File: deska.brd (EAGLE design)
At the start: 64.4 x 69.8 mm, 17 parts, among them X1 JST-XH-03-PIN-LONG-PAD

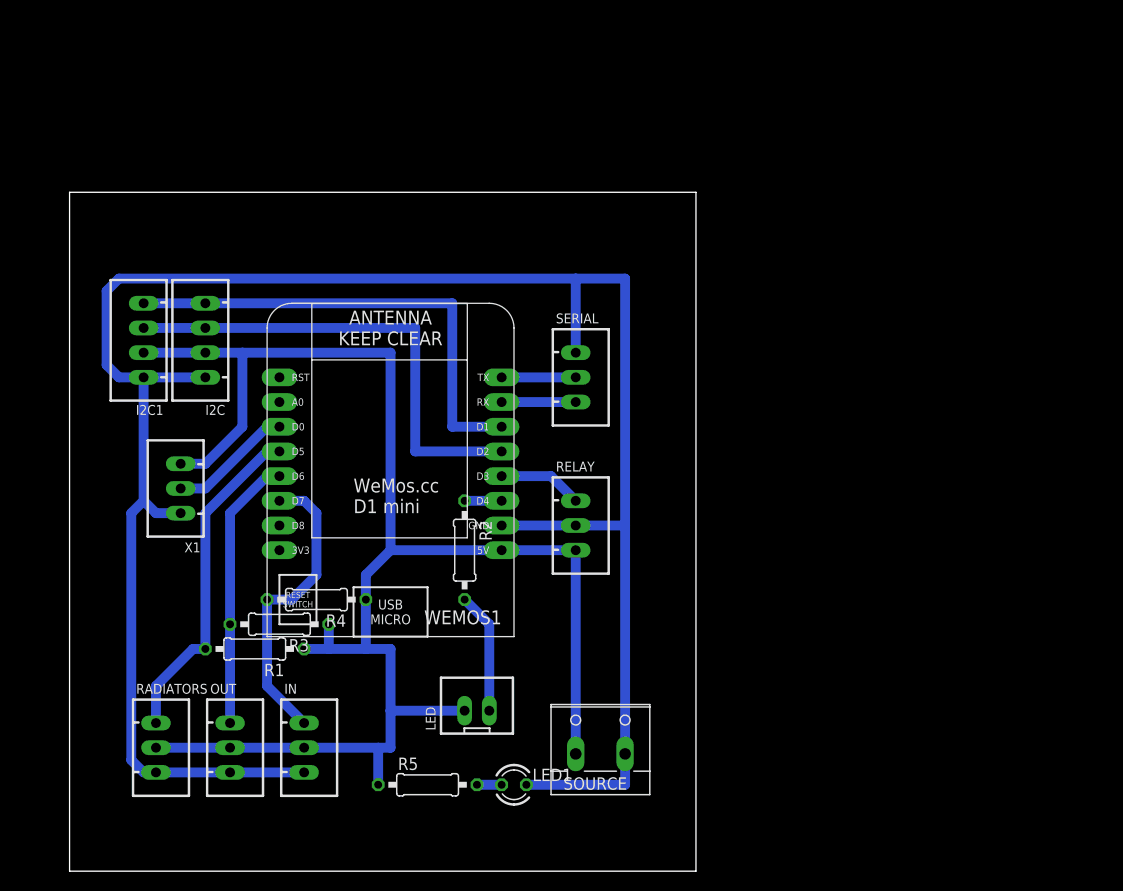
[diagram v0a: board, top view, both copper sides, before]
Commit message: +
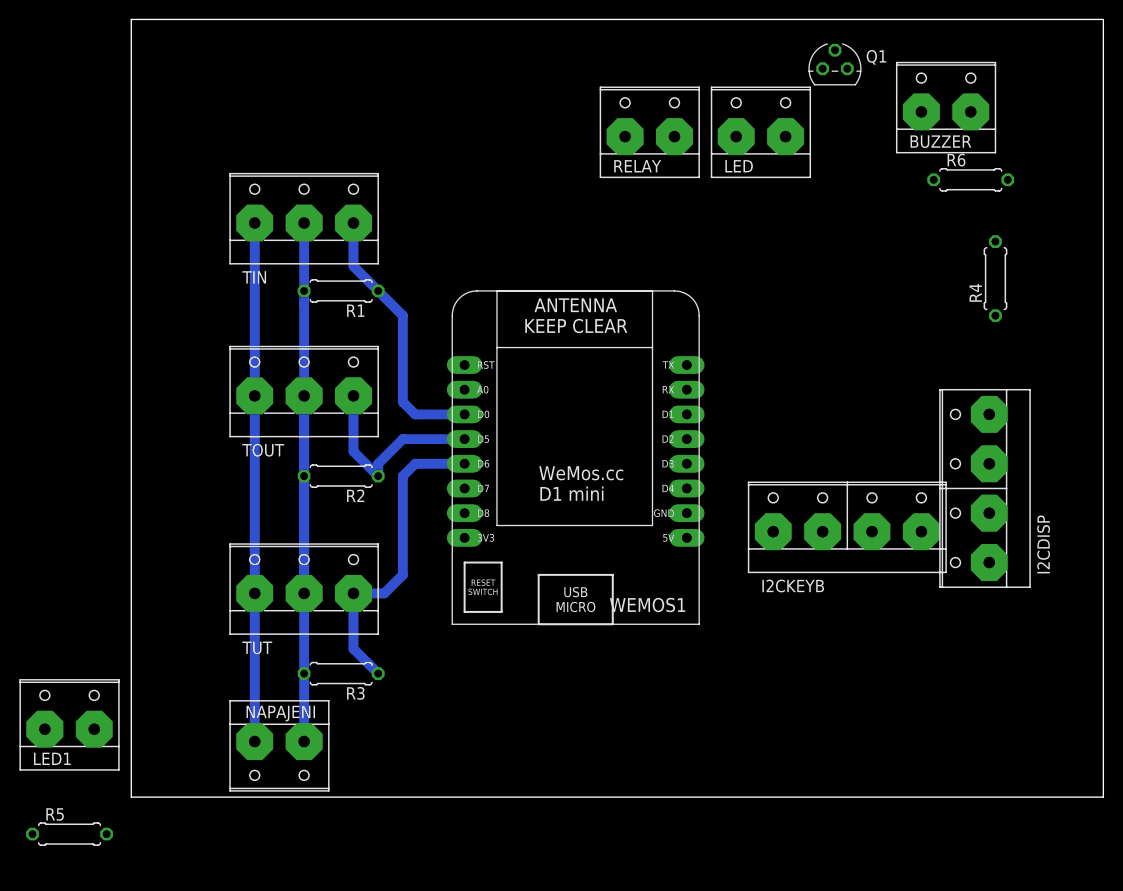
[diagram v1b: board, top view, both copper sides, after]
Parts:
- removed I2C, I2C1: JST-XH-04-PIN-LONG-PAD, Rembrandt Electronics - JST XH Connectors v1-0:JST-XH-04-PACKAGE-LONG-PAD
- removed IN, OUT, RADIATORS, SERIAL, X1: JST-XH-03-PIN-LONG-PAD, Rembrandt Electronics - JST XH Connectors v1-0:JST-XH-03-PACKAGE-LONG-PAD
- removed SOURCE: (no value), con-wago-508:W237-132
- added BUZZER, NAPAJENI: (no value), con-wago-508:W237-132
- added I2CDISP, I2CKEYB: (no value), con-wago-508:W237-4P
- added Q1: BC547, transistor-npn:TO92
- added R6: 1k, rcl:0207/7
- added TIN, TOUT, TUT: (no value), con-wago-508:W237-3E
- LED: value JST-XH-02-PIN-LONG-PAD -> (none); device Rembrandt Electronics - JST XH Connectors v1-0:JST-XH-02-PACKAGE-LONG-PAD -> con-wago-508:W237-132
- LED1: device led:LED3MM -> con-wago-508:W237-132
- R1, R3, R5: device rcl:0207/10 -> rcl:0207/7
- R2: value 220 -> 4k7; device rcl:0207/10 -> rcl:0207/7
- R4: value 4k7 -> 220; device rcl:0207/10 -> rcl:0207/7
- RELAY: value JST-XH-03-PIN-LONG-PAD -> (none); device Rembrandt Electronics - JST XH Connectors v1-0:JST-XH-03-PACKAGE-LONG-PAD -> con-wago-508:W237-132
- WEMOS1: device esp8266modules:WEMOS-D1-MINI -> wemos:WEMOS-D1-MINI
- moved R4 77.3 mm to (88.9, 53.3), turned to 90 degrees
- moved LED 66.5 mm to (64.8, 68.6)
- moved LED1 46.2 mm to (-6.35, 7.62)
- moved RELAY 41.3 mm to (53.3, 68.6), turned to 0 degrees
- moved R1 37.9 mm to (21.6, 52.1)
- moved R5 37.2 mm to (-6.35, -3.81)
- moved WEMOS1 19.1 mm to (44.5, 36.8)
- moved R2 14.8 mm to (21.6, 33.0), turned to 180 degrees
- moved R3 8.13 mm to (21.6, 12.7)
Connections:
- removed net N$10: LED1.A, R5.2
- removed net N$13: OUT.1, R3.2, WEMOS1.D6
- removed net N$4: I2C.3, I2C1.3, WEMOS1.D2
- removed net N$9: IN.1, R4.2, WEMOS1.D7
- new net N$12: I2CDISP.3, I2CKEYB.3, WEMOS1.D2
- new net N$14: R5.1, RELAY.1, WEMOS1.D3
- new net N$15: BUZZER.1, Q1.3
- new net N$19: R2.1, TOUT.3, WEMOS1.D5
- net +5V: now also I2CDISP.2, I2CKEYB.2, LED.2, LED1.1, NAPAJENI.1, R1.2, R2.2, R3.2, RELAY.2, TIN.2, TOUT.2, TUT.2; no longer I2C.2, I2C1.2, IN.2, LED.1, OUT.2, R1.1, R3.1, R4.1, R5.1, RADIATORS.2, RELAY.3, SOURCE.1, X1.3
- net GND: now also BUZZER.2, I2CDISP.1, I2CKEYB.1, NAPAJENI.2, Q1.1, TIN.1, TOUT.1, TUT.1; no longer I2C.1, I2C1.1, IN.3, LED1.K, OUT.3, RADIATORS.3, RELAY.2, SERIAL.1, SOURCE.2, X1.1
- net N$1: now also R1.1, TIN.3, WEMOS1.D0; no longer SERIAL.2, WEMOS1.TX
- net N$11: now also I2CDISP.4, I2CKEYB.4, WEMOS1.D1; no longer R1.2, RADIATORS.1, WEMOS1.D5
- net N$2: now also LED1.2, R5.2; no longer SERIAL.3, WEMOS1.RX
- net N$3: now also R3.1, TUT.3, WEMOS1.D6; no longer I2C.4, I2C1.4, WEMOS1.D1
- net N$5: now also R4.1, WEMOS1.D8; no longer WEMOS1.D0, X1.2
- net N$6: now also LED.1, R4.2; no longer R2.1, WEMOS1.D4
- net N$7: now also Q1.2, R6.1; no longer RELAY.1, WEMOS1.D3
- net N$8: now also R6.2, WEMOS1.D7; no longer LED.2, R2.2
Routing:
- net GND: track 217.3 -> 53.3 mm
- net +5V: track 169.6 -> 73.7 mm
- net N$4: track 49.5 -> 0.00 mm
- net N$11: track 34.7 -> 0.00 mm
- net N$9: track 31.1 -> 0.00 mm
- net N$13: track 28.2 -> 0.00 mm
- net N$19: track 0.00 -> 20.5 mm
- net N$1: track 7.62 -> 27.4 mm
- net N$3: track 49.5 -> 32.2 mm
- net N$5: track 12.8 -> 0.00 mm
- net N$8: track 12.5 -> 0.00 mm
- net N$7: track 8.67 -> 0.00 mm
- net N$2: track 7.62 -> 0.00 mm
- net N$6: track 3.81 -> 0.00 mm
- net N$10: track 2.54 -> 0.00 mm
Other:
- board size 64.4 x 69.8 mm -> 100 x 80 mm

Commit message: +
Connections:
- new net BUILTINLED: WEMOS1.D4
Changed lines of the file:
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@@
 <wire x1="34.29" y1="31.75" x2="90.17" y2="63.5" width="0" layer="19" extent="1-1"/>
+</signal>
+<signal name="BUILTINLED">
+<contactref element="WEMOS1" pad="D4"/>
 </signal>
 </signals>
